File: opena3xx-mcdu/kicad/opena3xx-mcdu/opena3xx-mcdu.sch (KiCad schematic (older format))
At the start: 50 parts, among them J1 Conn_02x01, J2 Conn_02x01, J3 Conn_02x01, J4 Conn_02x01, J5 Conn_02x01, J6 Conn_02x01, SW1 SW_MEC_5E, U1 MCP23017_SO, U2 MCP23017_SO, U3 MCP23017_SO, U4 MCP23017_SO, U5 MCP23017_SO

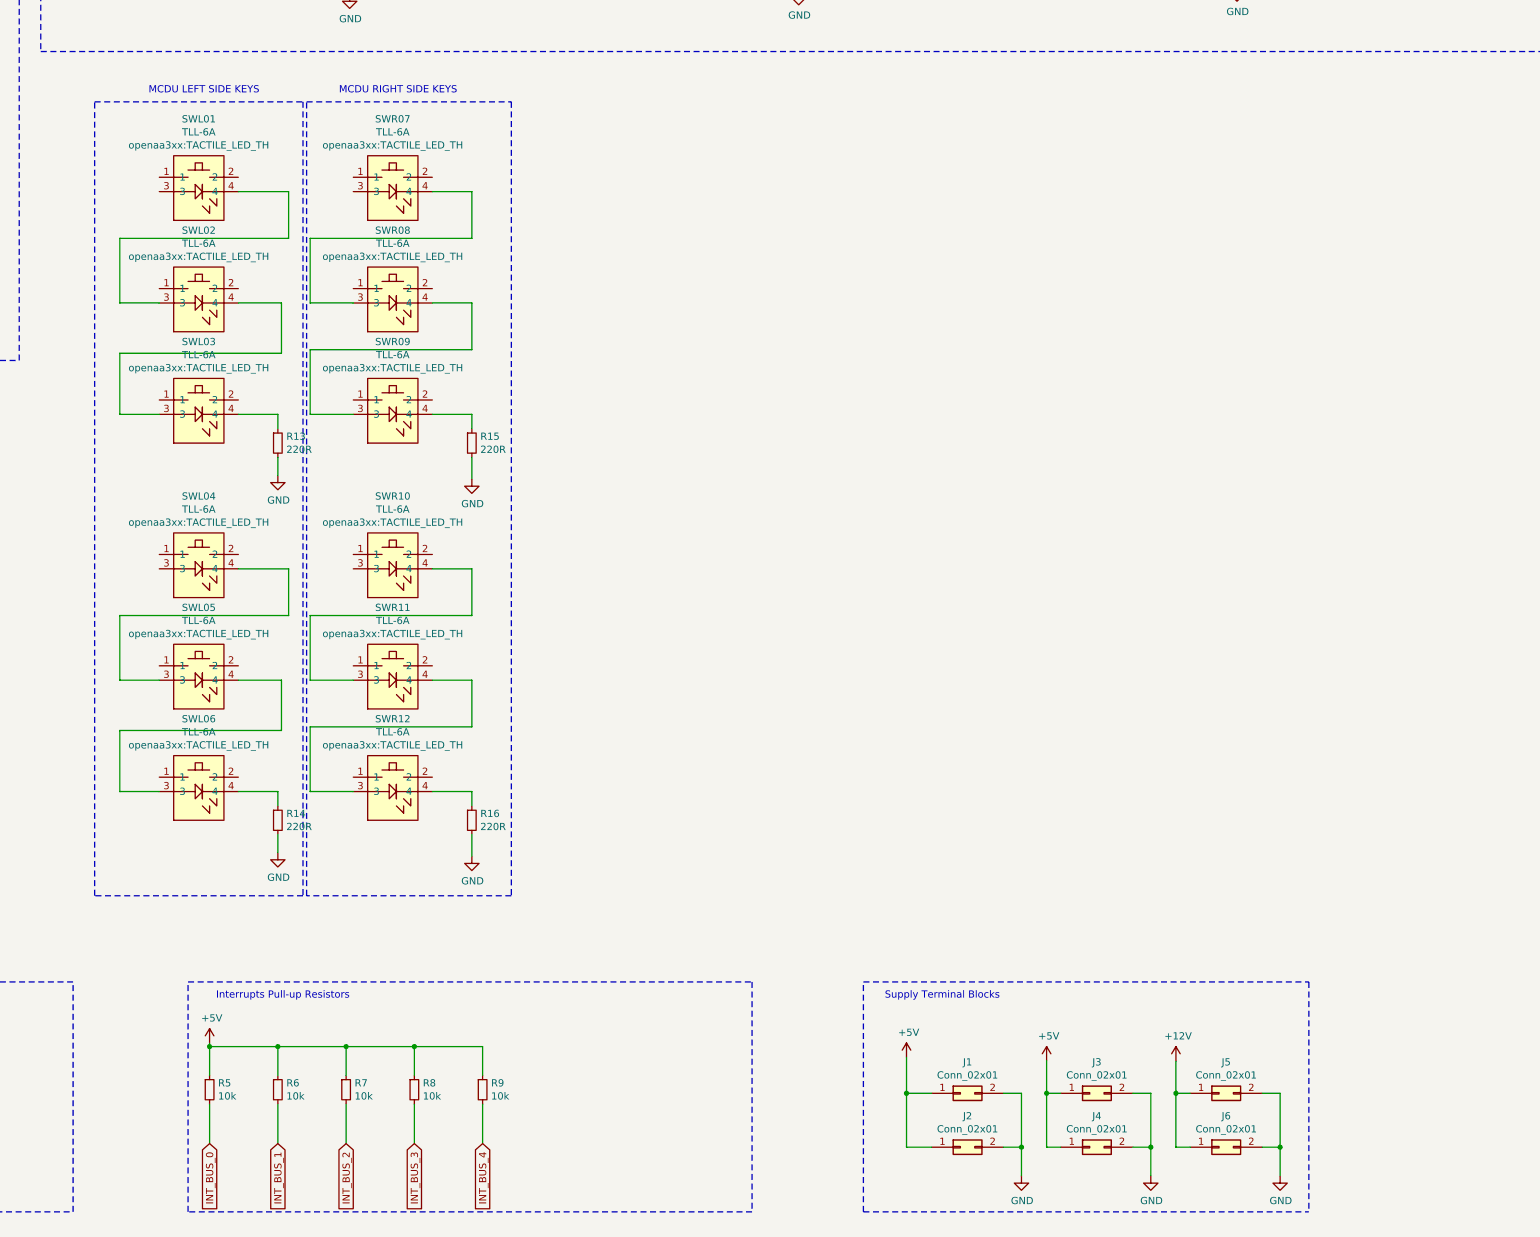
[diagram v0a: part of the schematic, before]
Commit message: MCDU Updates
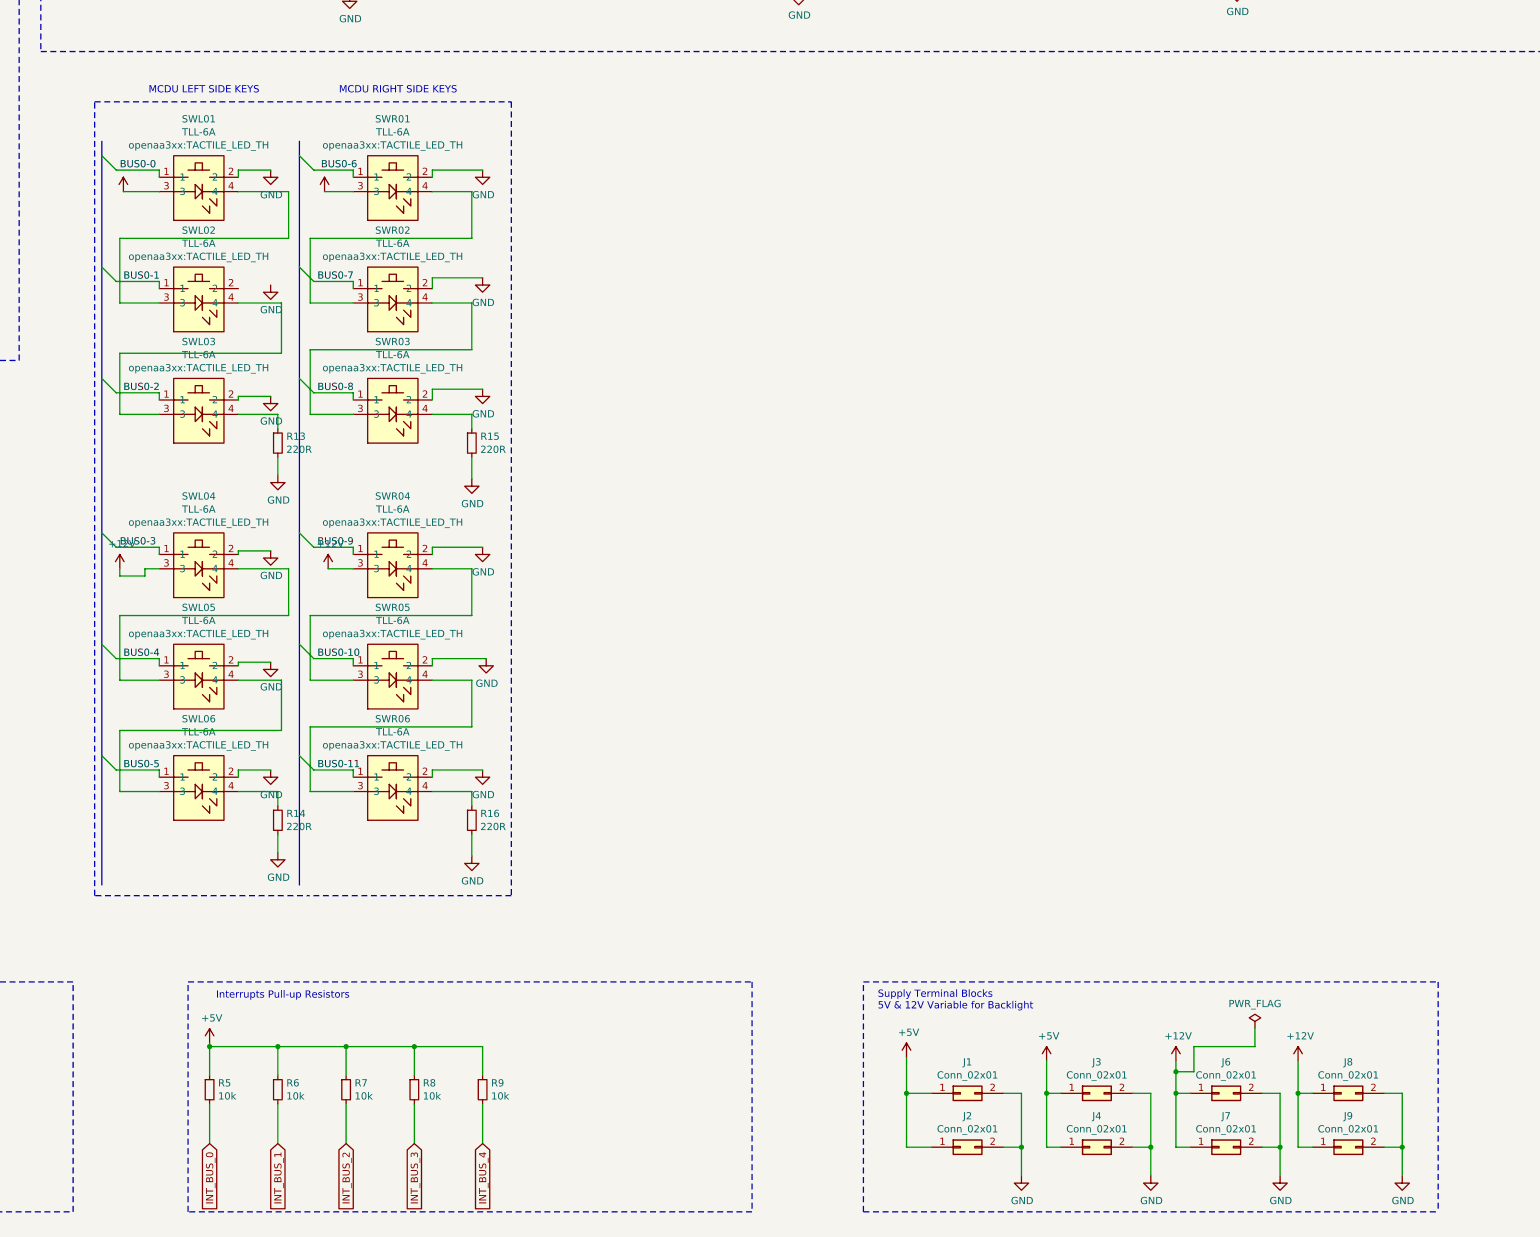
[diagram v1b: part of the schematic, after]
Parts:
- added J8, J9: Conn_02x01, TerminalBlock:TerminalBlock_bornier-2_P5.08mm, symbol Connector_Generic:Conn_02x01
- J5: footprint TerminalBlock:TerminalBlock_bornier-2_P5.08mm -> Connector_PinHeader_2.54mm:PinHeader_2x20_P2.54mm_Vertical
- R13, R14, R15, R16: footprint (none) -> Resistor_SMD:R_1210_3225Metric_Pad1.30x2.65mm_HandSolder
- renumbered J5 to J6, J6 to J7, SWR07 to SWR01, SWR08 to SWR02, SWR09 to SWR03, SWR10 to SWR04, SWR11 to SWR05, SWR12 to SWR06
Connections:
- net +12V: now also SWL01.3, SWL04.3, SWR01.3, SWR04.3, J8.1 (Pin_1), J9.1 (Pin_1)
- net BUS0-0: now also SWL01.1
- net BUS0-1: now also SWL02.1
- net BUS0-10: now also SWR05.1
- net BUS0-11: now also SWR06.1
- net BUS0-2: now also SWL03.1
- net BUS0-3: now also SWL04.1
- net BUS0-4: now also SWL05.1
- net BUS0-5: now also SWL06.1
- net BUS0-6: now also SWR01.1
- net BUS0-7: now also SWR02.1
- net BUS0-8: now also SWR03.1
- net BUS0-9: now also SWR04.1
- net GND: now also SWL01.2, SWL03.2, SWL04.2, SWL05.2, SWL06.2, SWR01.2, SWR02.2, SWR03.2, SWR04.2, SWR05.2, SWR06.2, J8.2 (Pin_2), J9.2 (Pin_2)
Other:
- note added: "Supply Terminal Blocks\n5V & 12V Variable for Backlight\n"
- note removed: "Supply Terminal Blocks\n"

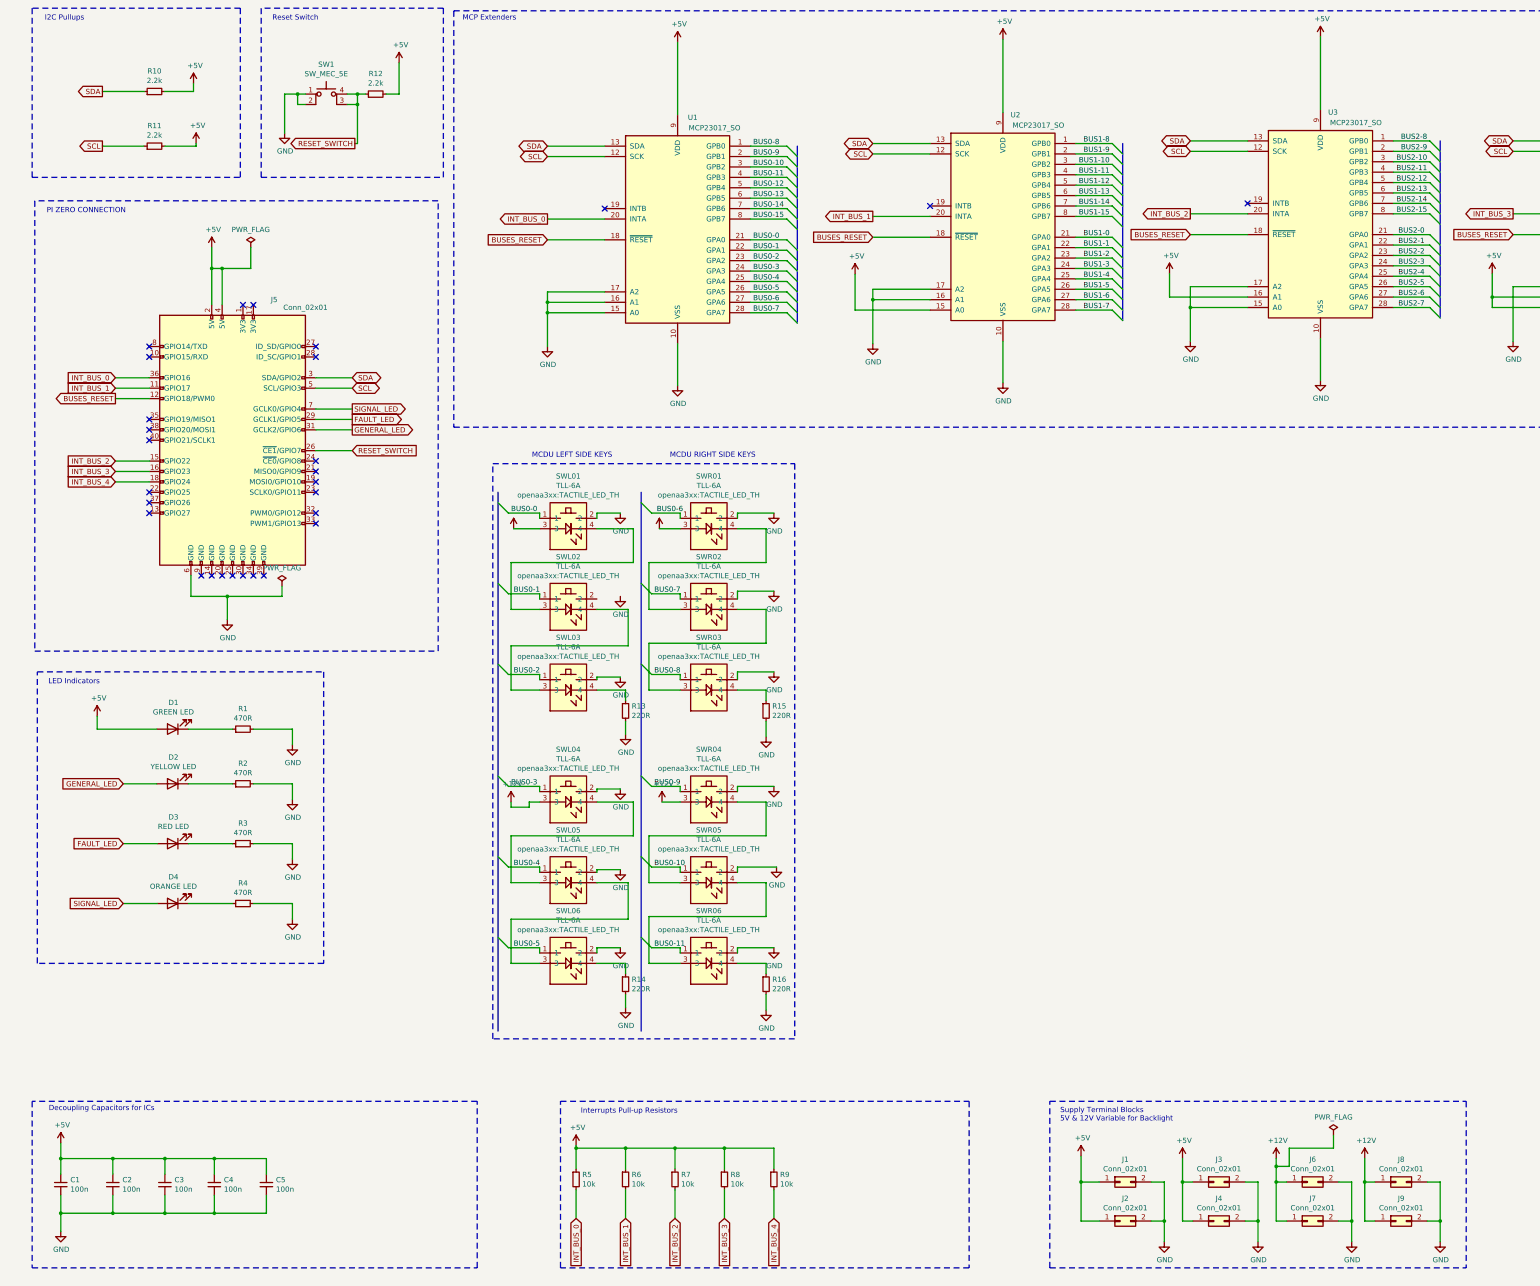
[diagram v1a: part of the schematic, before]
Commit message: Updates MCDU Schematic
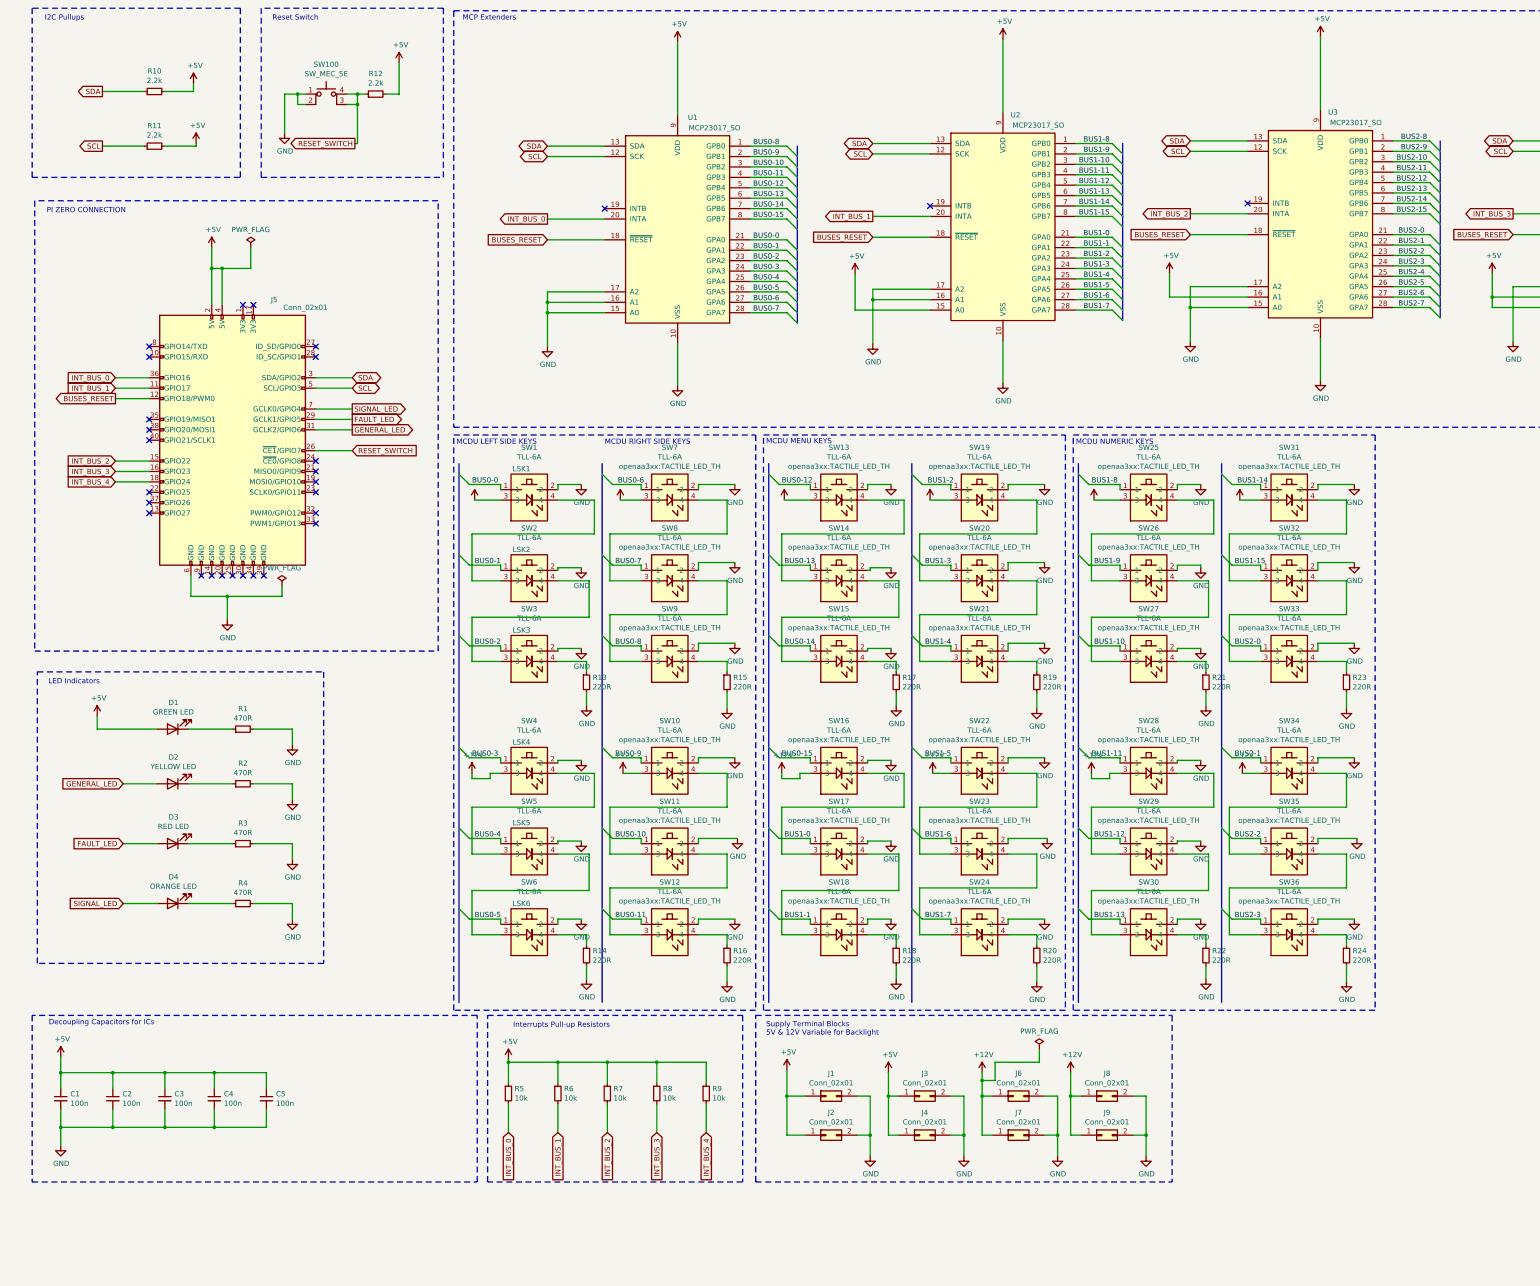
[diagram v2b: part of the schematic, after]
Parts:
- added R17, R18, R19, R20, R21, R22, R23, R24: 220R, Resistor_SMD:R_1210_3225Metric_Pad1.30x2.65mm_HandSolder, symbol Device:R_Small
- added SW13, SW14, SW15, SW16, SW17, SW18, SW19, SW20, SW21, SW22, SW23, SW24, SW25, SW26, SW27, SW28, SW29, SW30, SW31, SW32, SW33, SW34, SW35, SW36: TLL-6A, openaa3xx:TACTILE_LED_TH, symbol opena3xx-kicad:TLL-6A
- SW1: renamed from SWL01; MCDU IO Name (none) -> LSK1
- SW10: renamed from SWR04; MCDU IO Name (none) -> RSK4
- SW11: renamed from SWR05; MCDU IO Name (none) -> RSK5
- SW12: renamed from SWR06; MCDU IO Name (none) -> RSK6
- SW2: renamed from SWL02; MCDU IO Name (none) -> LSK2
- SW3: renamed from SWL03; MCDU IO Name (none) -> LSK3
- SW4: renamed from SWL04; MCDU IO Name (none) -> LSK4
- SW5: renamed from SWL05; MCDU IO Name (none) -> LSK5
- SW6: renamed from SWL06; MCDU IO Name (none) -> LSK6
- SW7: renamed from SWR01; MCDU IO Name (none) -> RSK1
- SW8: renamed from SWR02; MCDU IO Name (none) -> RSK2
- SW9: renamed from SWR03; MCDU IO Name (none) -> RSK3
- renumbered SW1 to SW100
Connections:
- net +12V: now also SW13.3, SW16.3, SW19.3, SW22.3, SW25.3, SW28.3, SW31.3, SW34.3
- net BUS0-12: now also SW13.1
- net BUS0-13: now also SW14.1
- net BUS0-14: now also SW15.1
- net BUS0-15: now also SW16.1
- net BUS1-0: now also SW17.1
- net BUS1-1: now also SW18.1
- net BUS1-10: now also SW27.1
- net BUS1-11: now also SW28.1
- net BUS1-12: now also SW29.1
- net BUS1-13: now also SW30.1
- net BUS1-14: now also SW31.1
- net BUS1-15: now also SW32.1
- net BUS1-2: now also SW19.1
- net BUS1-3: now also SW20.1
- net BUS1-4: now also SW21.1
- net BUS1-5: now also SW22.1
- net BUS1-6: now also SW23.1
- net BUS1-7: now also SW24.1
- net BUS1-8: now also SW25.1
- net BUS1-9: now also SW26.1
- net BUS2-0: now also SW33.1
- net BUS2-1: now also SW34.1
- net BUS2-2: now also SW35.1
- net BUS2-3: now also SW36.1
- net GND: now also SW2.2, R17.2, R18.2, R19.2, R20.2, R21.2, R22.2, R23.2, R24.2, SW13.2, SW14.2, SW15.2, SW16.2, SW17.2, SW18.2, SW19.2, SW20.2, SW21.2, SW22.2, SW23.2, SW24.2, SW25.2, SW26.2, SW27.2, SW28.2, SW29.2, SW30.2, SW31.2, SW32.2, SW33.2, SW34.2, SW35.2, SW36.2
- new net: SW19.4, SW20.3
- new net: SW20.4, SW21.3
- new net: R19.1, SW21.4
- new net: SW22.4, SW23.3
- new net: SW23.4, SW24.3
- new net: R20.1, SW24.4
- new net: R18.1, SW18.4
- new net: SW17.4, SW18.3
- new net: SW16.4, SW17.3
- new net: R17.1, SW15.4
- new net: SW14.4, SW15.3
- new net: SW13.4, SW14.3
- new net: SW31.4, SW32.3
- new net: SW32.4, SW33.3
- new net: R23.1, SW33.4
- new net: SW34.4, SW35.3
- new net: SW35.4, SW36.3
- new net: R24.1, SW36.4
- new net: R22.1, SW30.4
- new net: SW29.4, SW30.3
- new net: SW28.4, SW29.3
- new net: R21.1, SW27.4
- new net: SW26.4, SW27.3
- new net: SW25.4, SW26.3
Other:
- note added: "MCDU MENU KEYS\n\n"
- note added: "MCDU NUMERIC KEYS\n"
- moved on the sheet: C1, C2, C3, C4, C5, J1, J2, J3, J4, J6, J7, J8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
